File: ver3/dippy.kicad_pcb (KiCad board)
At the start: 2 copper layers, 29.5 x 68.7 mm, 24 parts, among them J1 Conn_01x02_Female, J2 Screw_Terminal_01x03, J3 Screw_Terminal_01x04, J4 Conn_Coaxial, J5 Conn_02x03_Odd_Even, U1 ATmega328P-PU-C, U2 RFM95W-915S2, U3 MCP1700-3302E_SOT23, Y1 Crystal

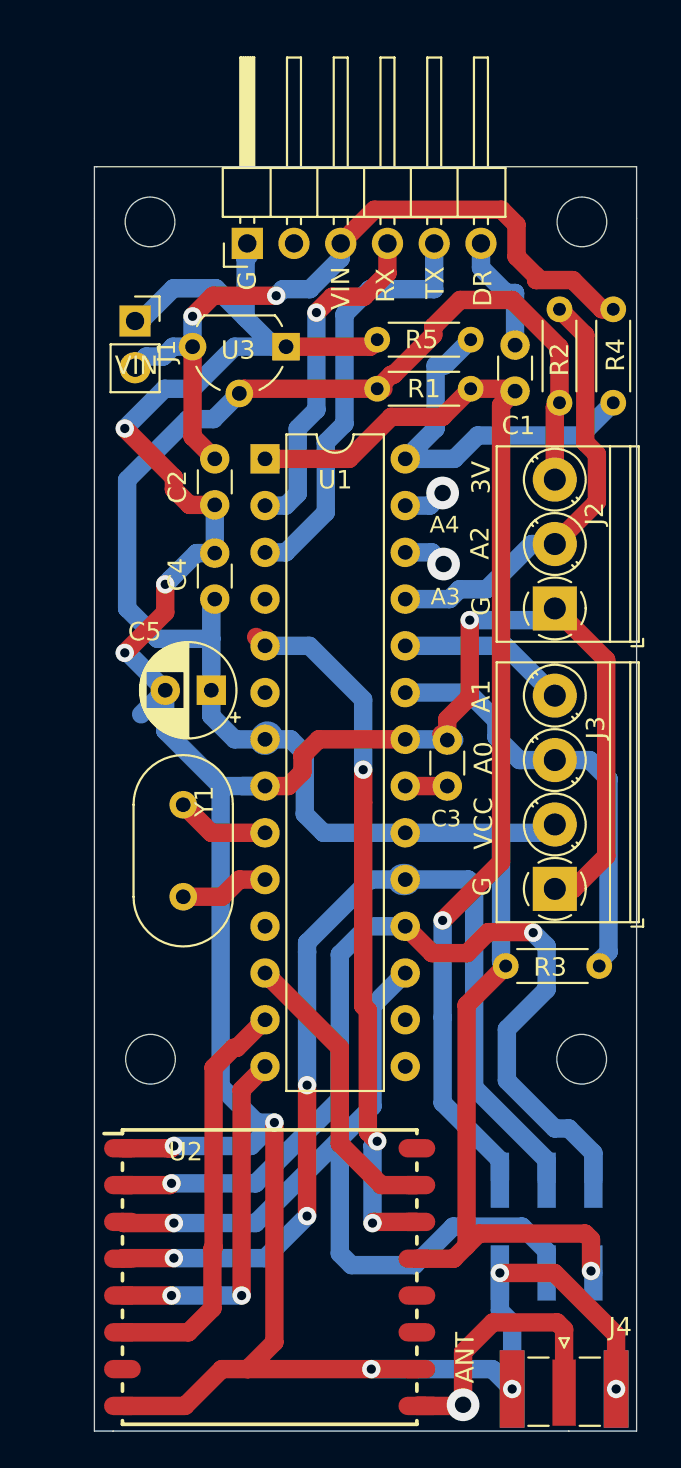
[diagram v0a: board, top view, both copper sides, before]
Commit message: update
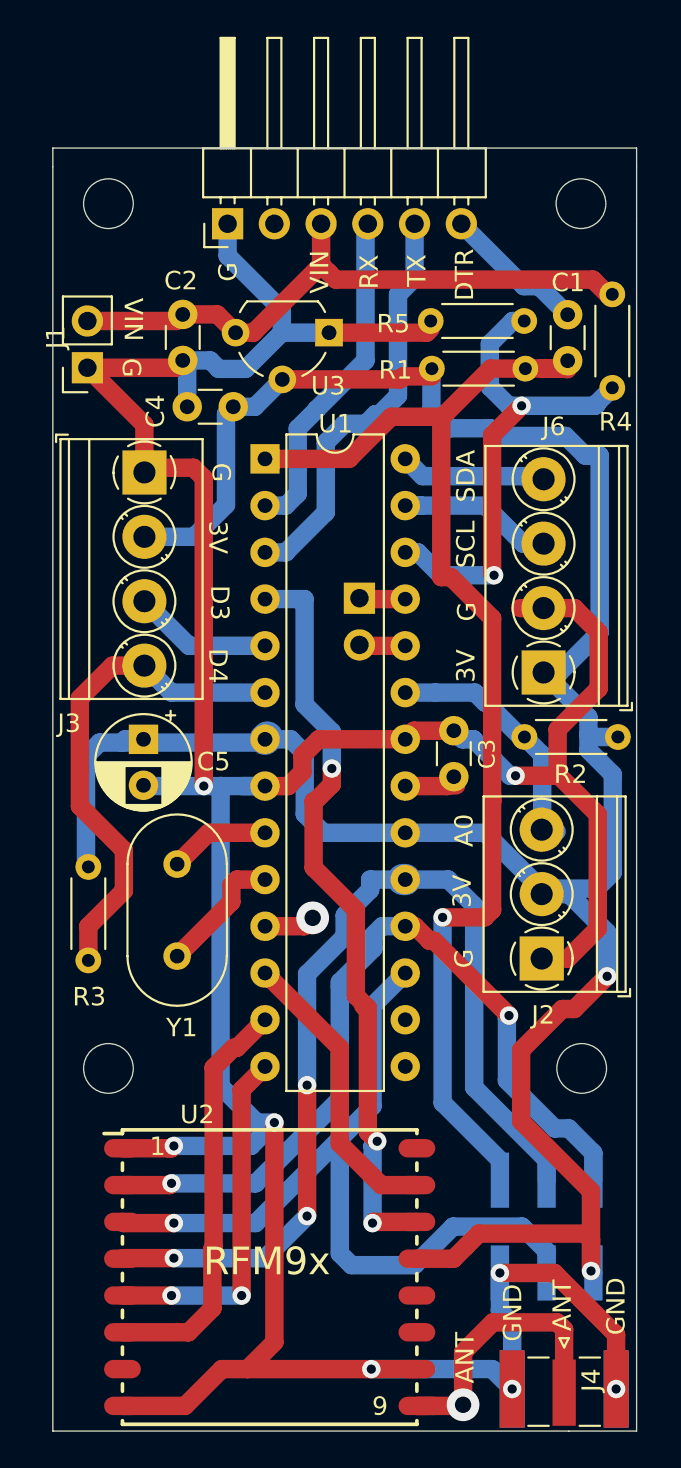
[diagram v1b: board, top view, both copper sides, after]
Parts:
- added J6: Screw_Terminal_01x04, TerminalBlock_Phoenix:TerminalBlock_Phoenix_PT-1,5-4-3.5-H_1x04_P3.50mm_Horizontal, F.Cu at (140.9, 91.0)
- added J7: Conn_01x02_Female, Connector_PinSocket_2.54mm:PinSocket_1x02_P2.54mm_Vertical, B.Cu at (130.9, 86.9)
- moved J3 31.8 mm to (119.2, 80.1), turned to 270 degrees
- moved R3 23.3 mm to (116.1, 101.5), turned to 270 degrees
- moved J2 19.0 mm to (140.8, 106.5)
- moved R2 18.4 mm to (144.9, 94.5), turned to 180 degrees
- moved C4 10.5 mm to (124.0, 76.5), turned to 180 degrees
- moved C2 8.04 mm to (121.3, 71.5)
- moved C5 4.55 mm to (119.1, 94.6), turned to 270 degrees
- moved J1 3.63 mm to (116.1, 74.4), turned to 180 degrees
- moved C1 3.30 mm to (142.2, 74.0)
- moved Y1 3.24 mm to (121.0, 101.4)
- moved R1 3.17 mm to (134.8, 74.5)
- moved R5 3.08 mm to (139.8, 71.9)
- moved H4 2.47 mm to (117.2, 65.5)
- moved U3 2.46 mm to (129.2, 72.5)
- moved H2 2.34 mm to (117.2, 112.5)
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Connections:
- J2 pad 2: A2 -> VCC
- J2 pad 3: VCC -> A0
- J3 pad 3: A0 -> D3
- J3 pad 4: A1 -> D4
- R2 pad 2: A2 -> A0
- R3 pad 2: A0 -> D4
- R4 pad 2: A5 -> A3
- R5 pad 1: A5 -> A3
- U1 pad 26: (no net) -> A3
- U1 pad 27: (no net) -> A4
- U1 pad 4: (no net) -> D2
- U1 pad 6: (no net) -> D4
- U2 pad 14: D3 -> D2
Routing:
- net D2: track 0.00 -> 41.5 mm, vias 0 -> 3
- net D3: track 38.5 -> 7.56 mm, vias 3 -> 0
- net VCC: track 114.6 -> 144.6 mm, vias 1 -> 2
- net A3: track 0.00 -> 27.5 mm, vias 0 -> 2
- net D4: track 0.00 -> 27.4 mm
- net A2: track 23.9 -> 2.51 mm
- net A5: track 20.8 -> 7.98 mm
- net A0: track 24.1 -> 13.9 mm
- net A4: track 0.00 -> 9.37 mm
- net GND: track 189.6 -> 198.3 mm, vias 10 -> 8
- net VIN: track 41.0 -> 33.5 mm, vias 2 -> 0
- net MISO: track 51.3 -> 44.4 mm
- net A1: track 9.38 -> 2.51 mm
- net Net-(C1-Pad1): track 61.0 -> 65.8 mm
- net Net-(U1-Pad10): track 4.83 -> 7.03 mm
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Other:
- board size 29.5 x 68.7 mm -> 31.7 x 69.7 mm
- board text added: "1"
- board text added: "9"
- board text added: "D3"
- board text added: "D4"
- board text added: "D5"
- board text added: "DTR"
- board text added: "GND"
- board text added: "MI"
- board text added: "MO"
- board text added: "RFM9x"
- board text added: "RST"
- board text added: "SCK"
- board text added: "SCL"
- board text added: "SDA"
- board text removed: "A3"
- board text removed: "A4"
- board text removed: "DR"
- board text removed: "VCC"
